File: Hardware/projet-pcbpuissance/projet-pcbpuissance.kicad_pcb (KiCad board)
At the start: 2 copper layers, 83.8 x 61 mm, 35 parts, among them J2 Conn_01x02, J3 Conn_01x02, J4 Conn_01x02, U1 MAX5033DUSA+, U2 MAX5033DUSA+

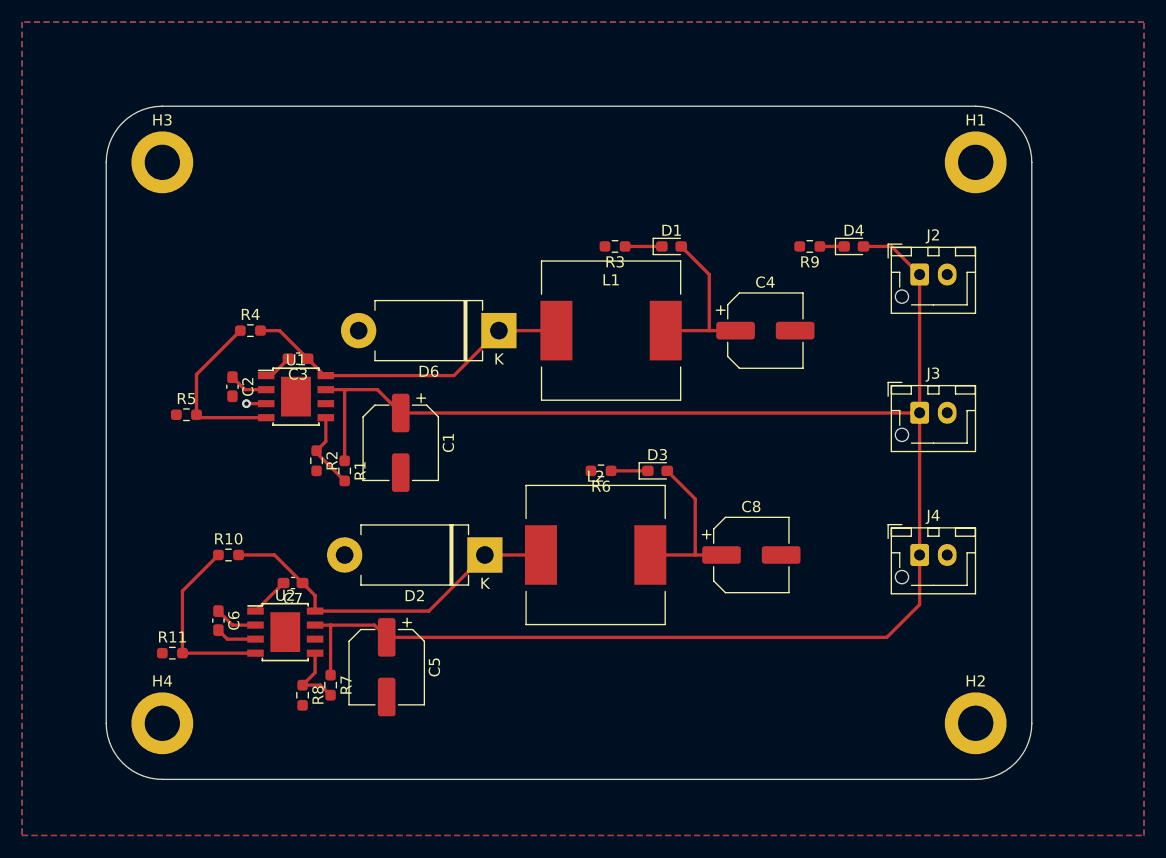
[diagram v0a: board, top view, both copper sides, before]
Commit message: Modif pcb puissance
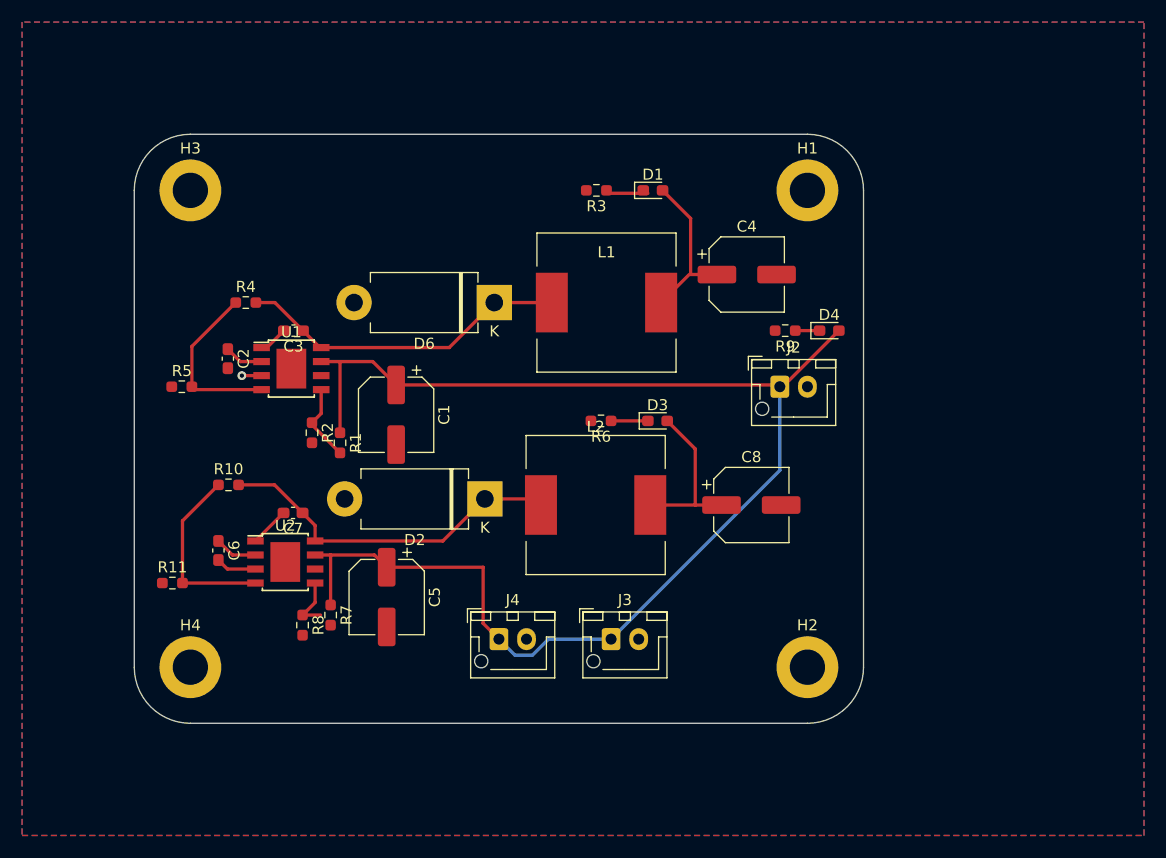
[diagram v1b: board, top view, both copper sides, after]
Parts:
- moved J4 38.9 mm to (122.8, 108.5)
- moved J3 34.7 mm to (133.0, 108.5)
- moved J2 16.2 mm to (148.3, 85.6)
- moved H2 16.1 mm to (150.8, 111.0)
- moved H1 15.5 mm to (150.8, 67.8)
- moved R9 7.94 mm to (148.8, 80.5)
- moved D4 7.94 mm to (152.7, 80.5)
- moved R10 6.35 mm to (98.3, 94.5)
- moved R11 6.35 mm to (93.3, 103.4)
- moved U2 6.35 mm to (103.5, 101.5)
- moved C5 6.35 mm to (112.7, 104.7)
- moved C6 6.35 mm to (97.4, 100.5)
- moved C7 6.35 mm to (104.2, 97.1)
- moved R7 6.35 mm to (107.6, 106.3)
- moved R8 6.35 mm to (105.1, 107.2)
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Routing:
- net Batterie 11.1 V: track 158.1 -> 124.2 mm
- net Net-(U2-ON/~{OFF}): track 6.29 -> 5.00 mm
- net Net-(D2-K): track 32.4 -> 33.2 mm
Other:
- board size 83.8 x 61 mm -> 66 x 53.3 mm
